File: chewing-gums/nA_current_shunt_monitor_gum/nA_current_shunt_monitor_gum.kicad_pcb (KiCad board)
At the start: 4 copper layers, 15.2 x 27.9 mm, 34 parts, among them IC6 INA212AIDCKR, J1 Conn_Coaxial, J2 Conn_01x03, J3 Conn_01x03, J6 Conn_02x01, J7 Conn_02x01, U1 TLV75801PDBV, U2 ADS1219, U3 TLV75801PDBV, U4 MCP4726, U5 24AA02E-OT

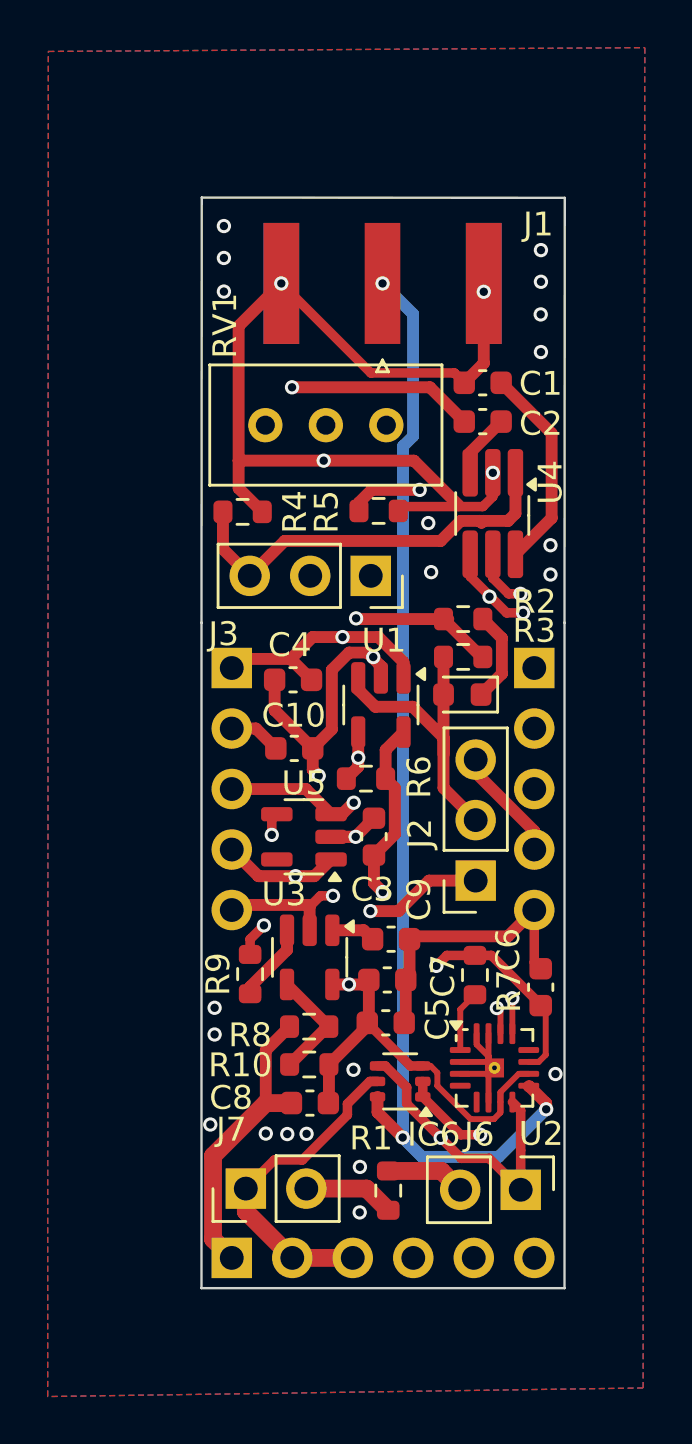
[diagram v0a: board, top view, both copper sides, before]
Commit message: production files
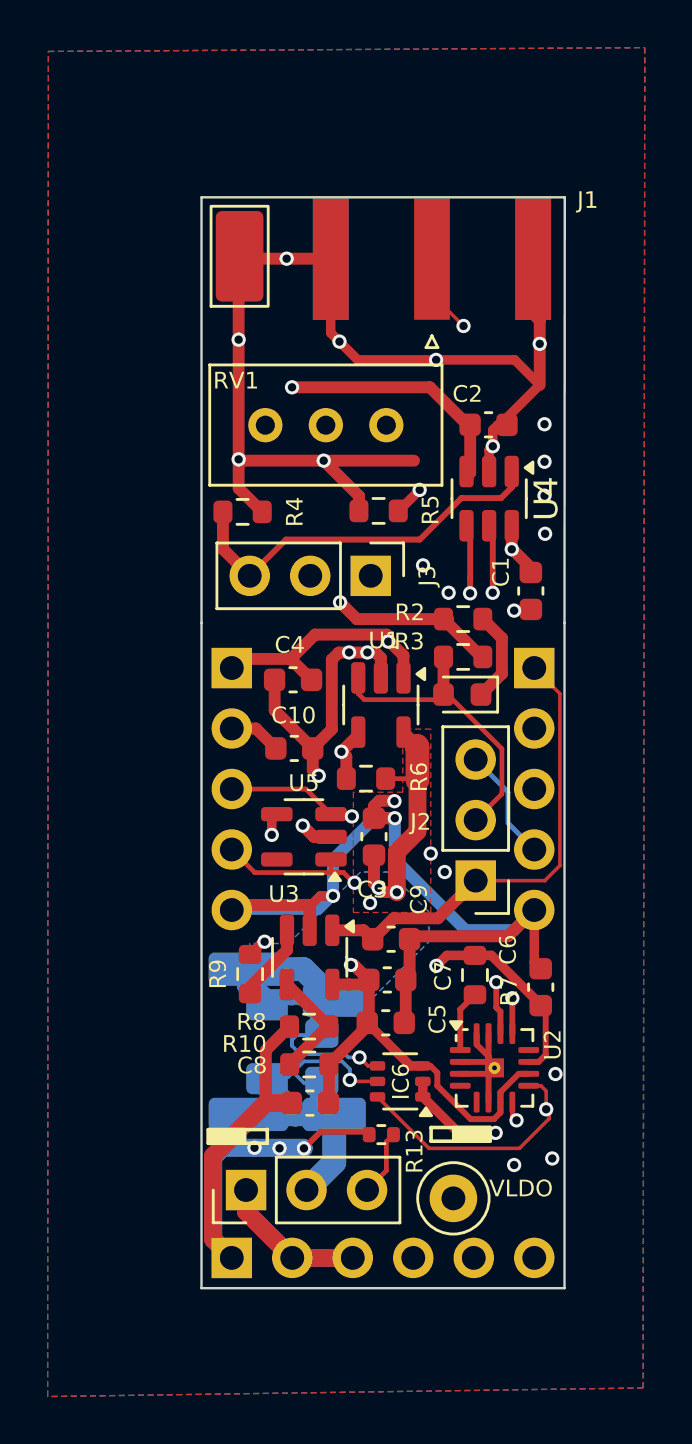
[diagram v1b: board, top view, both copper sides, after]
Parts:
- removed J6: Conn_02x01, Connector_PinHeader_2.54mm:PinHeader_1x02_P2.54mm_Vertical
- added G***: LOGO, heep-footprints:EPFL_3x1, B.Cu at (126.7, 79.4)
- added G***: LOGO, heep-footprints:ESL_3x3, B.Cu at (131.3, 105.7)
- added R11: 10, Resistor_SMD:R_2010_5025Metric_Pad1.40x2.65mm_HandSolder, B.Cu at (127.6, 102.8)
- added R12: 10, Resistor_SMD:R_1206_3216Metric_Pad1.30x1.75mm_HandSolder, B.Cu at (124.8, 102.2)
- added R13: 1M, Resistor_SMD:R_0402_1005Metric, F.Cu at (129.6, 106.1)
- added R14: 10, Resistor_SMD:R_2512_6332Metric_Pad1.40x3.35mm_HandSolder, B.Cu at (124.0, 102.2)
- added TP14: 5029, TestPoint:TestPoint_Keystone_5019_Miniature, F.Cu at (123.7, 69.2)
- added TP2: ~, TestPoint:TestPoint_Loop_D1.80mm_Drill1.0mm_Beaded, F.Cu at (132.6, 108.8)
- J2, J3: footprint Connector_PinSocket_2.54mm:PinSocket_1x03_P2.54mm_Vertical -> Connector_PinHeader_2.54mm:PinHeader_1x03_P2.54mm_Vertical
- J7: footprint Connector_PinHeader_2.54mm:PinHeader_1x02_P2.54mm_Vertical -> Connector_PinHeader_2.54mm:PinHeader_1x03_P2.54mm_Vertical
- R1: footprint Resistor_SMD:R_0603_1608Metric -> Resistor_SMD:R_0805_2012Metric_Pad1.20x1.40mm_HandSolder; moved to B.Cu
- U4: footprint Package_TO_SOT_SMD:TSOT-23-6_HandSoldering -> Package_TO_SOT_SMD:TSOT-23-6
- moved C1 8.97 mm to (135.9, 83.2), turned to -90 degrees
- moved R1 6.26 mm to (127.1, 102.8)
- moved J1 2.31 mm to (131.7, 69.3)
- moved U4 0.64 mm to (134.1, 79.4)
- moved C2 0.28 mm to (134.1, 76.3), turned to 0 degrees
- moved J7 0.06 mm to (123.9, 108.4)
- turned R5 to 180 degrees
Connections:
- C1 pad 1: Net-(U4-Vref) -> A3.3V
- C2 pad 1: Net-(U4-VDD) -> 3.3V
- C2 pad 2: 3.3V -> GND
- C9 pad 1: Net-(U3-IN) -> /5V
- IC6 pad 5: /V_LSL_load -> /Shunt-
- J2 pad 1: A3.3V -> /5V
- J7 pad 2: Net-(J7-Pin_2) -> /Shunt-
- R1 pad 1: Net-(J7-Pin_2) -> /Shunt-
- R1 pad 2: Net-(J6-Pin_2) -> /V_LSL_LDO
- U3 pad 1: Net-(U3-IN) -> /5V
- U4 pad 3: Net-(U4-VDD) -> 3.3V
- U4 pad 6: Net-(U4-Vref) -> A3.3V
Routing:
- net GND: track 127.5 -> 162.3 mm, vias 31 -> 30
- net /5V: track 19.0 -> 37.3 mm
- net /Shunt-: track 0.00 -> 18.1 mm, vias 0 -> 1
- net A3.3V: track 26.0 -> 42.9 mm
- net /V_LSL_load: track 13.9 -> 28.5 mm
- net /V_LSL_LDO: track 31.9 -> 43.2 mm, vias 2 -> 5
- net Net-(U4-Vref): track 8.72 -> 0.00 mm
- net /SDA: track 38.6 -> 34.2 mm
- net Net-(J7-Pin_2): track 3.82 -> 0.00 mm
- net Net-(J7-Pin_3): track 0.00 -> 3.59 mm
- net Net-(J6-Pin_2): track 3.35 -> 0.00 mm
- net Net-(U4-VDD): track 2.72 -> 0.00 mm
- net /ADC0: track 47.2 -> 49.5 mm, vias 3 -> 2
- net 3.3V: track 54.5 -> 56.6 mm
- net Net-(U3-IN): track 1.85 -> 0.00 mm
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- added copper zone on B.Cu, net /V_LSL_LDO
- added copper zone on F.Cu, net /V_LSL_LDO
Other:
- board text added: "ESL 2025"
- board text added: "I-trace output"
- board text added: "INA21[x]"
- board text added: "Programmable supply & current monitor"
- board text added: "SHUNT R (Ohms)"
- board text added: "VLDO"
- board text added: "x=[0|1|2|3|4|5]"
